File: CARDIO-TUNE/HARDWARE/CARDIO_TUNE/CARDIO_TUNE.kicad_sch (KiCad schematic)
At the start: 13 parts, among them J1 TPA, J2 MAX30102, J3 Screw_Terminal_01x02, SW1 SW_Nidec_CAS-120A1, SW2 SW_Push, U1 ESP32-DEVKITC

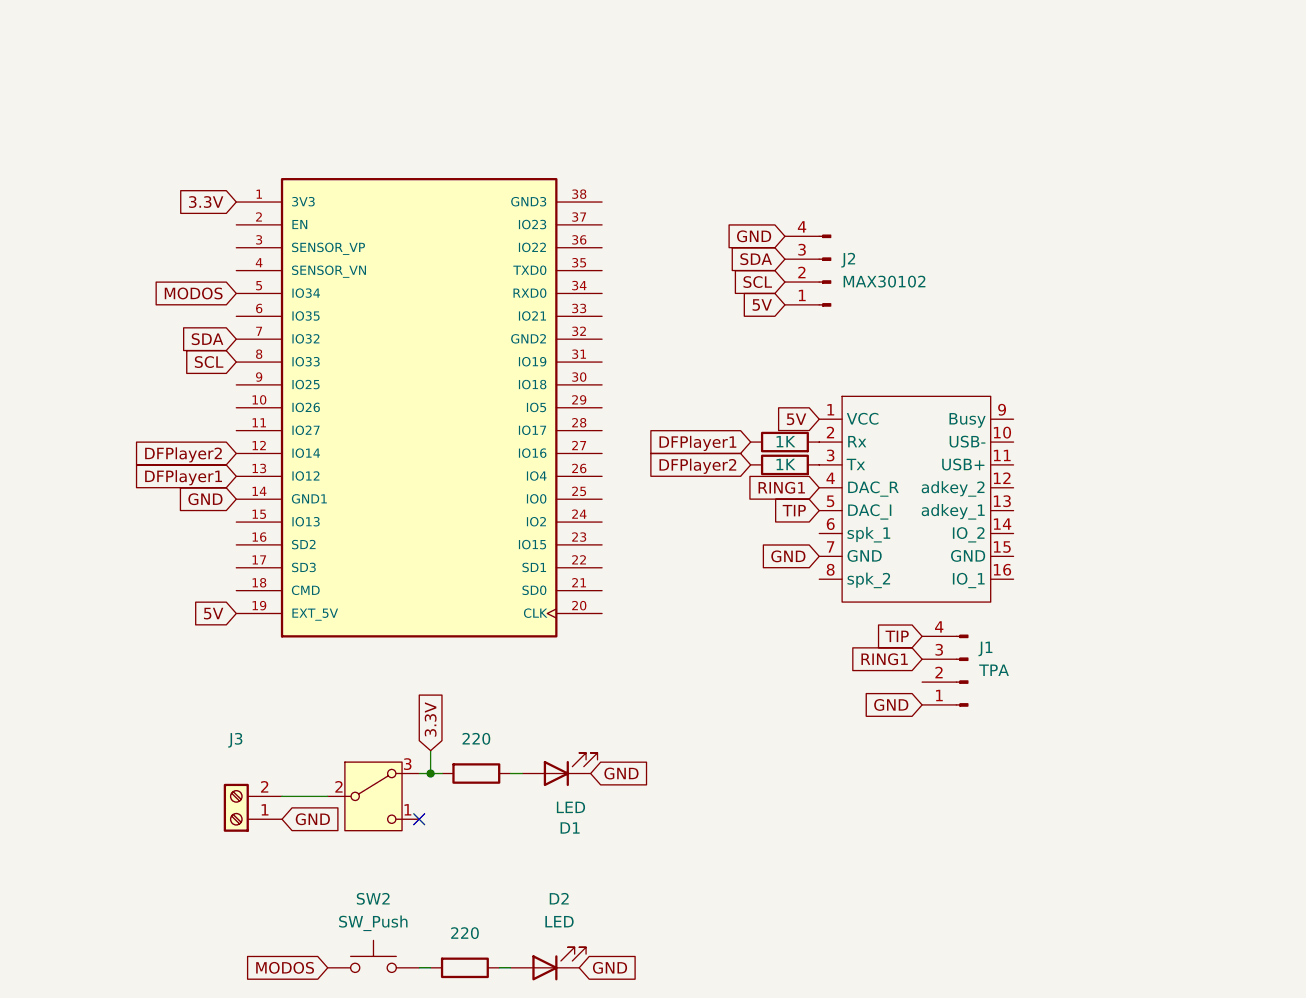
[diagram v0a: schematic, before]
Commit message: Add files via upload
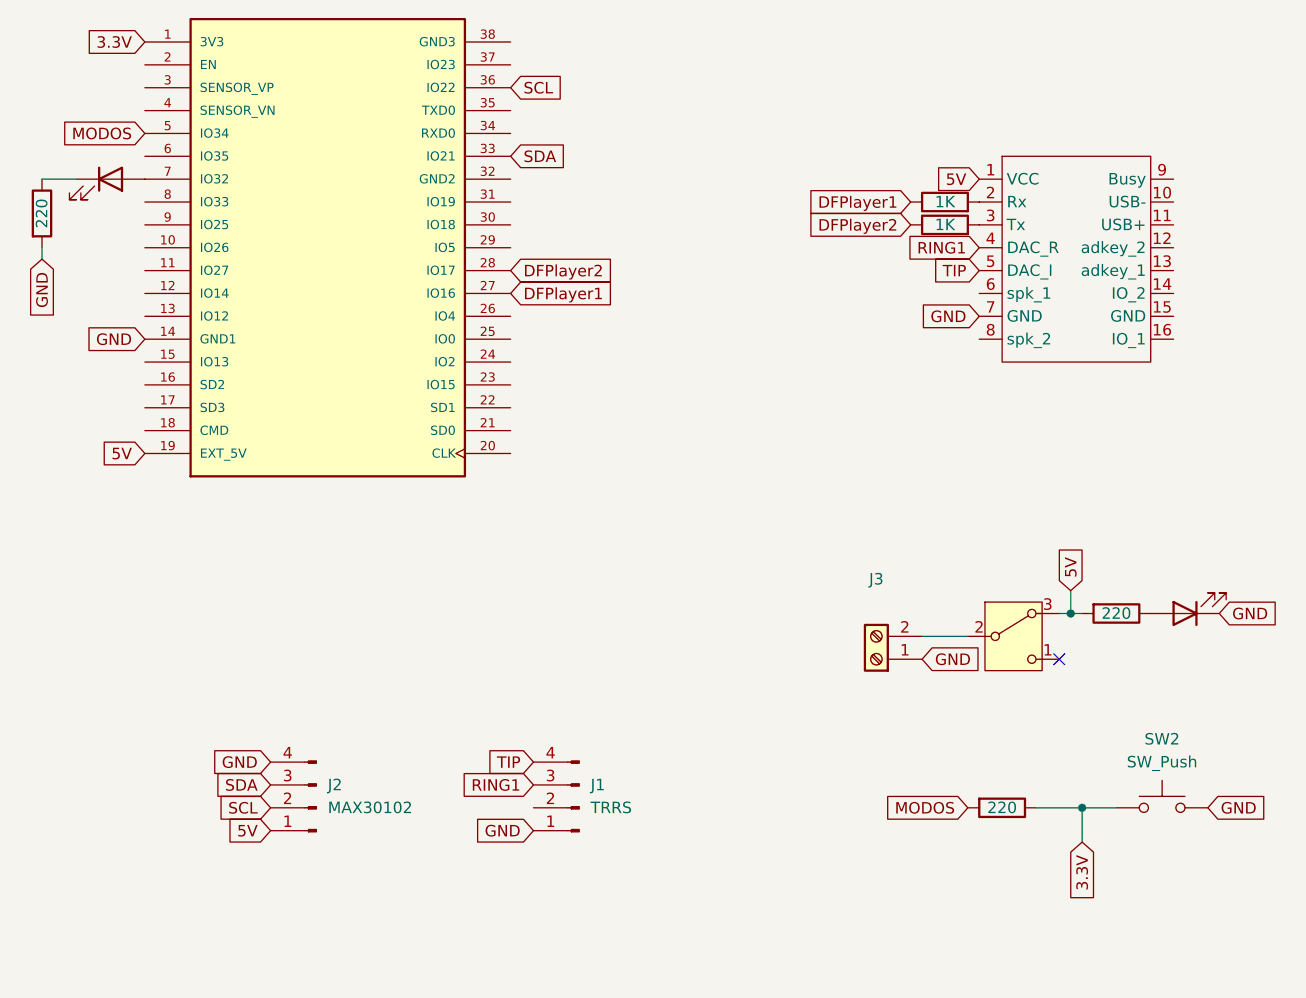
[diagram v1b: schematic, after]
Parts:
- added R5: 220, Resistor_THT:R_Axial_DIN0207_L6.3mm_D2.5mm_P7.62mm_Horizontal, symbol Device:R
- J1: value TPA -> TRRS
- SW1: footprint Button_Switch_SMD:Nidec_Copal_CAS-120A -> Connector_PinHeader_2.54mm:PinHeader_2x01_P2.54mm_Vertical
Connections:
- net 3.3V: now also R4.1, SW2.1; no longer R3.2, SW1.3 (A)
- net 5V: now also R3.2, SW1.3 (A)
- net DFPlayer1: now also U1.27 (IO16); no longer U1.13 (IO12)
- net DFPlayer2: now also U1.28 (IO17); no longer U1.12 (IO14)
- net GND: now also SW2.2, R5.2; no longer D2.1 (K)
- net MODOS: now also R4.2; no longer SW2.1
- net SCL: now also U1.36 (IO22); no longer U1.8 (IO33)
- net SDA: now also U1.33 (IO21); no longer U1.7 (IO32)
- net at D2.2 (A): now also U1.7 (IO32); no longer R4.1
- new net: D2.1 (K), R5.1
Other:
- moved on the sheet: J1, J2, J3, SW2

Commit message: Add files via upload
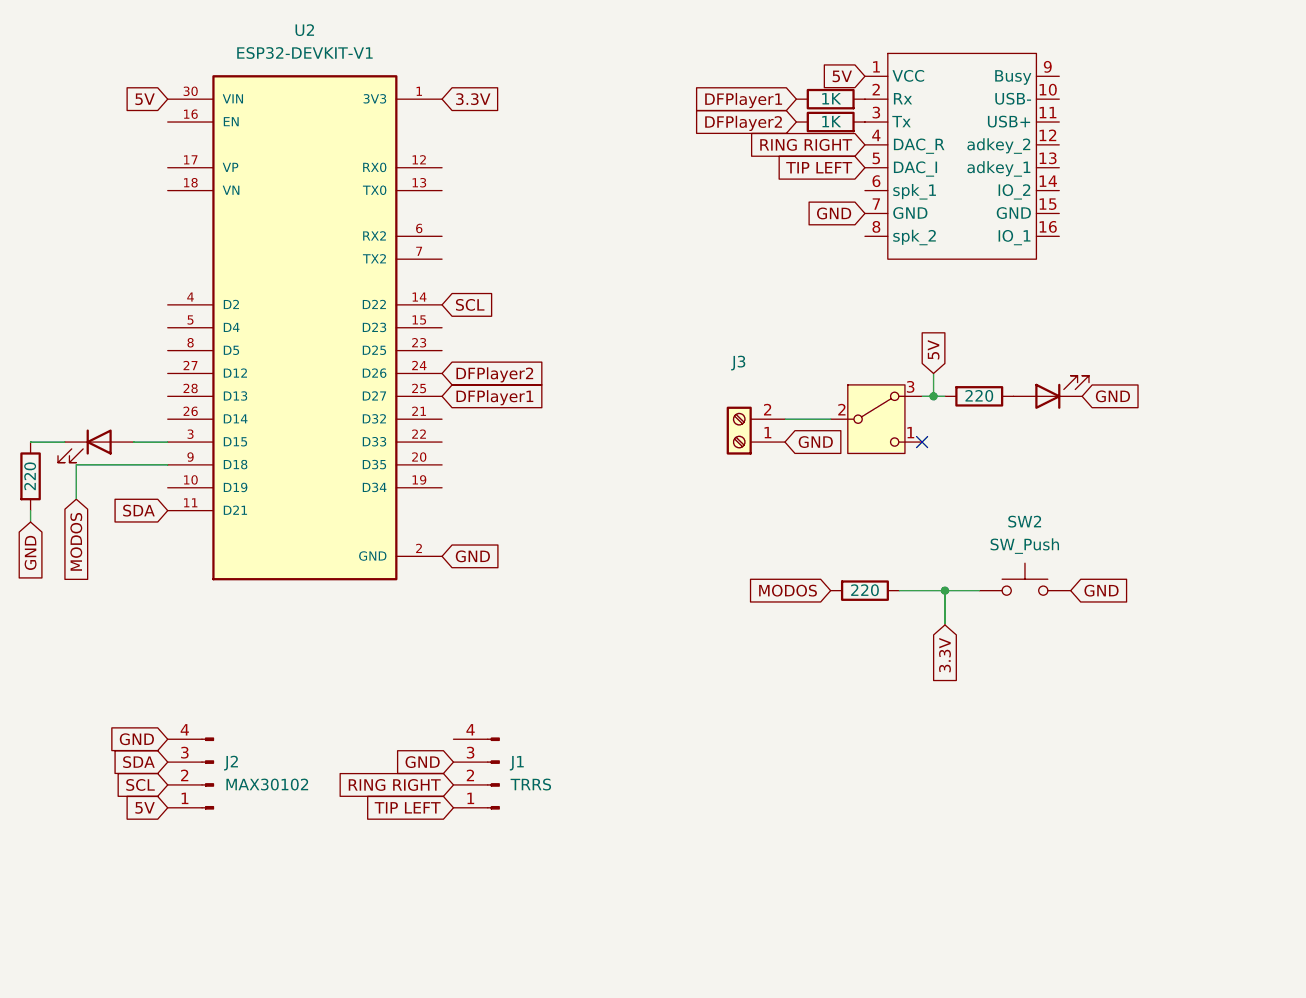
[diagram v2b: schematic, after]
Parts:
- removed D2: LED, LED_THT:LED_Rectangular_W3.0mm_H2.0mm, symbol Device:LED
- removed R5: 220, Resistor_THT:R_Axial_DIN0207_L6.3mm_D2.5mm_P7.62mm_Horizontal, symbol Device:R
- removed U1: ESP32-DEVKITC, HUELLAS:MODULE_ESP32-DEVKITC, symbol SIMBOLOS:ESP32-DEVKITC
- added D3: LED, LED_THT:LED_Rectangular_W3.0mm_H2.0mm, symbol Device:LED
- added R6: 220, Resistor_THT:R_Axial_DIN0207_L6.3mm_D2.5mm_P7.62mm_Horizontal, symbol Device:R
- added U2: ESP32-DEVKIT-V1, RF_Module:MODULE_ESP32_DEVKIT_V1, symbol ESP32-DEVKIT-V1:ESP32-DEVKIT-V1
- SW1: footprint Connector_PinHeader_2.54mm:PinHeader_2x01_P2.54mm_Vertical -> Connector_PinSocket_2.54mm:PinSocket_1x02_P2.54mm_Vertical
- U3: value ~ -> (none)
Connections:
- net 3.3V: now also U2.1 (3V3)
- net 5V: now also U2.30 (VIN)
- net DFPlayer1: now also U2.25 (D27)
- net DFPlayer2: now also U2.24 (D26)
- net GND: now also J1.3 (Pin_3), R6.2, U2.2 (GND), U2.29 (GND); no longer J1.1 (Pin_1)
- net MODOS: now also U2.9 (D18)
- net SCL: now also U2.14 (D22)
- net SDA: now also U2.11 (D21)
- net RING RIGHT: now reaches J1.2 (Pin_2)
- net RING RIGHT: now also U3.4 (DAC_R)
- removed net RING1: J1.3 (Pin_3), U3.4 (DAC_R)
- net TIP: no longer names the net of J1.4 (Pin_4)
- net TIP: no longer U3.5 (DAC_I)
- new net: D3.2 (A), U2.3 (D15)
- new net: D3.1 (K), R6.1
- new net TIP LEFT: J1.1 (Pin_1), U3.5 (DAC_I)
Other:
- moved on the sheet: J1, J2, J3, SW2
